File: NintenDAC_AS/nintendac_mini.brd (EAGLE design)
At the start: 25 x 50 mm, 21 parts, among them IC1 STM32F10XCXT6, IC3 24C64ST, X1 USB-MICROB

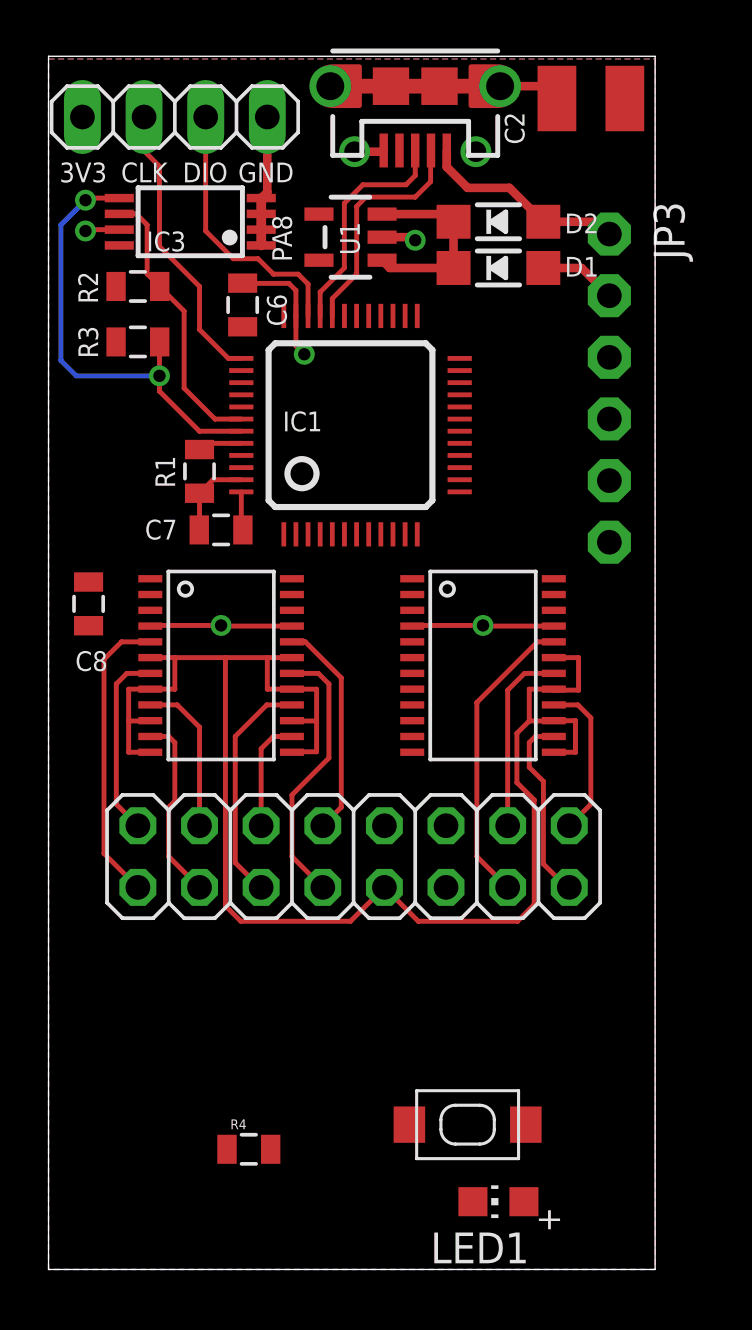
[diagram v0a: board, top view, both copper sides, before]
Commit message: continue working on AS
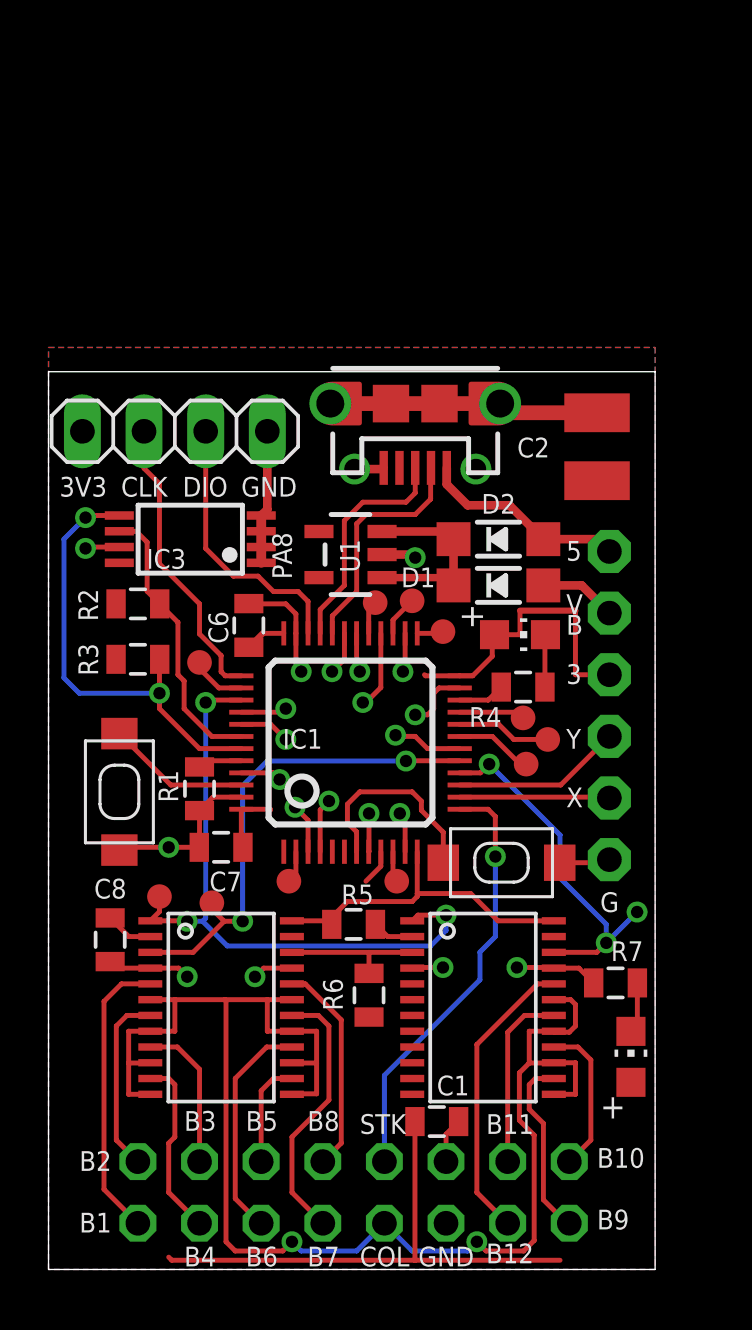
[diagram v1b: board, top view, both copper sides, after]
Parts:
- added C1: (no value), backplane:0805
- added LED2: (no value), adafruit:CHIP-LED0805
- added R5, R6, R7: (no value), SparkFun-Passives:0805
- added S2: SWITCH-MOMENTARY-2TURTLE, Adafruit Feather M0 Adalogger:KMR2
- added TP1, TP10, TP12, TP14, TP16, TP17, TP19, TP2, TP20, TP23, TP8, TP9: TEST-POINTTP_15TH_THRU, pth testpoint:TP_15TH
- added TP11, TP13, TP15, TP18, TP21, TP22, TP3, TP4, TP5, TP6, TP7: TEST-POINT3X4, SparkFun-Connectors:PAD.03X.04
- JP2: device pinhead:2X08 -> pinheadwerew:2X08
- moved LED1 23.4 mm to (19.4, 26.2), turned to 270 degrees
- moved R4 22.2 mm to (19.6, 24.0)
- moved C2 14.4 mm to (22.6, 33.9), turned to 90 degrees
- moved U$3 14.1 mm to (7.11, 10.8)
- moved U$4 14.1 mm to (17.9, 10.8)
- moved C8 13.9 mm to (2.54, 13.6)
- moved JP2 13.8 mm to (12.6, 3.17)
- moved C6 13.2 mm to (8.26, 26.5)
- moved IC1 13.1 mm to (12.4, 21.7)
- moved JP3 13.1 mm to (23.1, 23.2)
- moved U1 13.1 mm to (12.4, 29.5)
- moved X1 13.1 mm to (15.1, 35.7)
- moved C7 13.1 mm to (7.11, 17.4)
- moved D1 13.1 mm to (18.5, 28.2)
- moved D2 13.1 mm to (18.5, 30.1)
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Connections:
- removed net VBAT: IC1.1
- new net N$10: IC1.31, TP1.P$1
- new net N$11: IC1.20, TP4.P$1
- new net N$12: IC1.19, TP5.P$1
- new net N$13: IC1.21, TP3.P$1
- new net N$14: IC1.38, TP6.P$1
- new net N$15: IC1.2, TP7.P$1
- new net N$16: IC1.3, TP8.P$1
- new net N$17: IC1.4, TP9.P$1
- new net N$18: IC1.45, TP10.P$1
- new net N$19: IC1.29, TP11.P$1
- new net N$20: IC1.28, TP12.P$1
- new net N$21: IC1.27, TP13.P$1
- new net N$22: IC1.26, TP14.P$1
- new net N$23: IC1.25, TP15.P$1
- new net N$24: IC1.18, TP16.P$1
- new net N$25: IC1.10, TP18.P$1
- new net N$26: IC1.11, TP17.P$1
- new net N$27: IC1.40, TP20.P$1
- new net N$28: IC1.41, TP19.P$1
- new net N$29: LED2.C, R7.2
- new net N$5: R6.1, U$3.22, U$4.3
- new net N$6: IC1.30, TP2.P$1
- new net SPI1_CS: IC1.12, R5.1, U$3.24, U$4.24
- new net USER_BUTTON: IC1.46, S2.1
- new net USER_LED: IC1.22, R4.1
- net +3V3: now also C1.1, IC1.1, JP3.3, LED2.A, R5.2, R6.2, U$3.23, U$4.23; no longer JP3.6
- net GND: now also C1.2, JP3.6, R7.1, S2.3; no longer JP3.3, R4.1
- net SPI1_MISO: now also TP23.P$1; no longer U$3.22
- net SPI1_MOSI: now also TP21.P$1; no longer U$4.3
- net SPI1_SCK: now also TP22.P$1
- net STK: now also IC1.13
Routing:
- net +3V3: track 1.60 -> 44.1 mm
- net SPI1_SCK: track 0.00 -> 26.7 mm, vias 0 -> 3
- net SPI1_MOSI: track 0.00 -> 20.3 mm, vias 0 -> 2
- net STK: track 0.00 -> 17.7 mm, vias 0 -> 1
- net SPI1_MISO: track 0.00 -> 14.9 mm, vias 0 -> 2
- net SPI1_CS: track 0.00 -> 13.8 mm
- net GND: track 39.3 -> 50.1 mm, vias 5 -> 10
- net N$1: track 0.00 -> 8.45 mm
- net POTY: track 0.00 -> 7.00 mm
- net POTX: track 0.00 -> 6.18 mm
- net USER_BUTTON: track 0.00 -> 5.90 mm
- net N$5: track 0.00 -> 5.83 mm
- net N$11: track 0.00 -> 3.89 mm
- net N$20: track 0.00 -> 3.23 mm
- net N$12: track 0.00 -> 3.21 mm
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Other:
- board size 25 x 50 mm -> 25 x 37 mm
- board text added: "3"
- board text added: "5"
- board text added: "B1"
- board text added: "B10"
- board text added: "B11"
- board text added: "B12"
- board text added: "B2"
- board text added: "B3"
- board text added: "B4"
- board text added: "B5"
- board text added: "B6"
- board text added: "B7"
- board text added: "B8"
- board text added: "B9"
- board text added: "COL"
- board text added: "G"
- board text added: "STK"
- board text added: "V B"
- board text added: "X"
- board text added: "Y"
